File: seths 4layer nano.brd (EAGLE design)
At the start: 20.9 x 51.1 mm, 30 parts, among them IC1 FT232RL, J1 1981568-1, Q1 CSTCR6M00G53Z, X1 TSW-115-07-G-S, X2 TSW-115-07-G-S

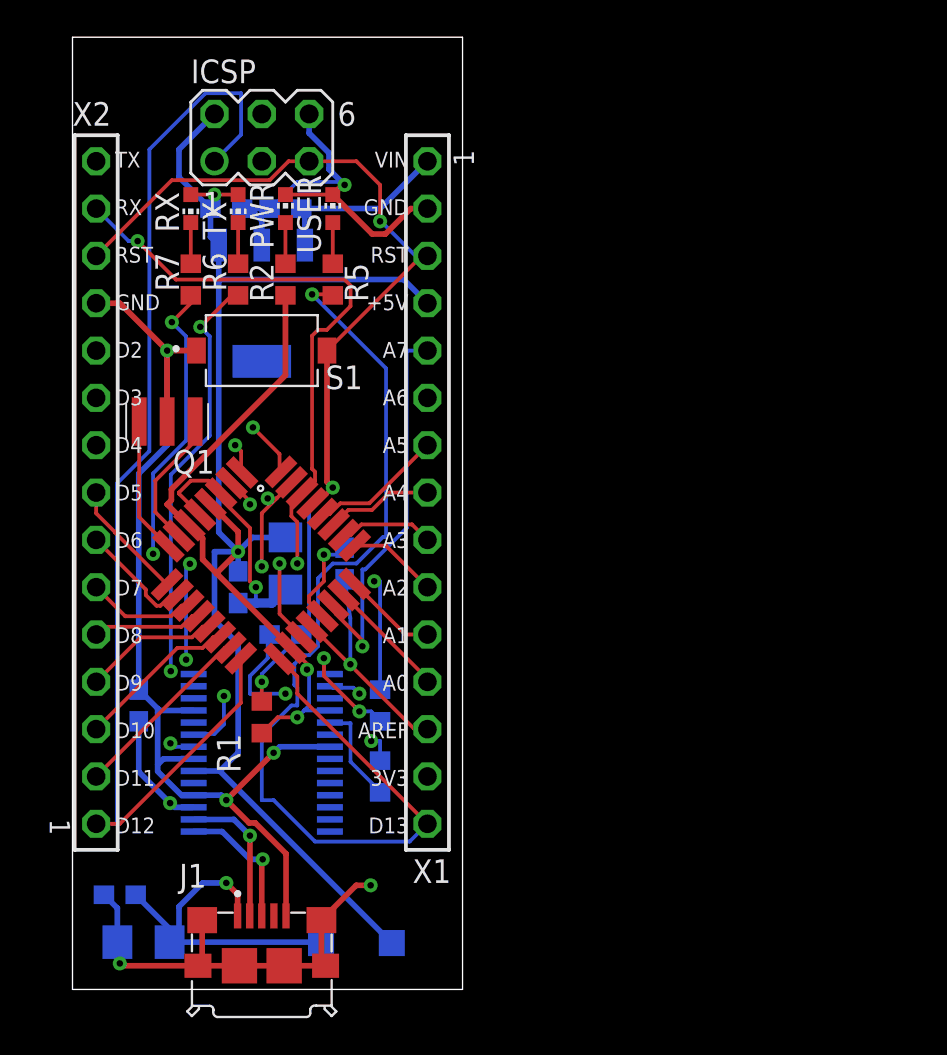
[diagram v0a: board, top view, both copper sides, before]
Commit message: Add files via upload
updating this since it hasn't been in a while.
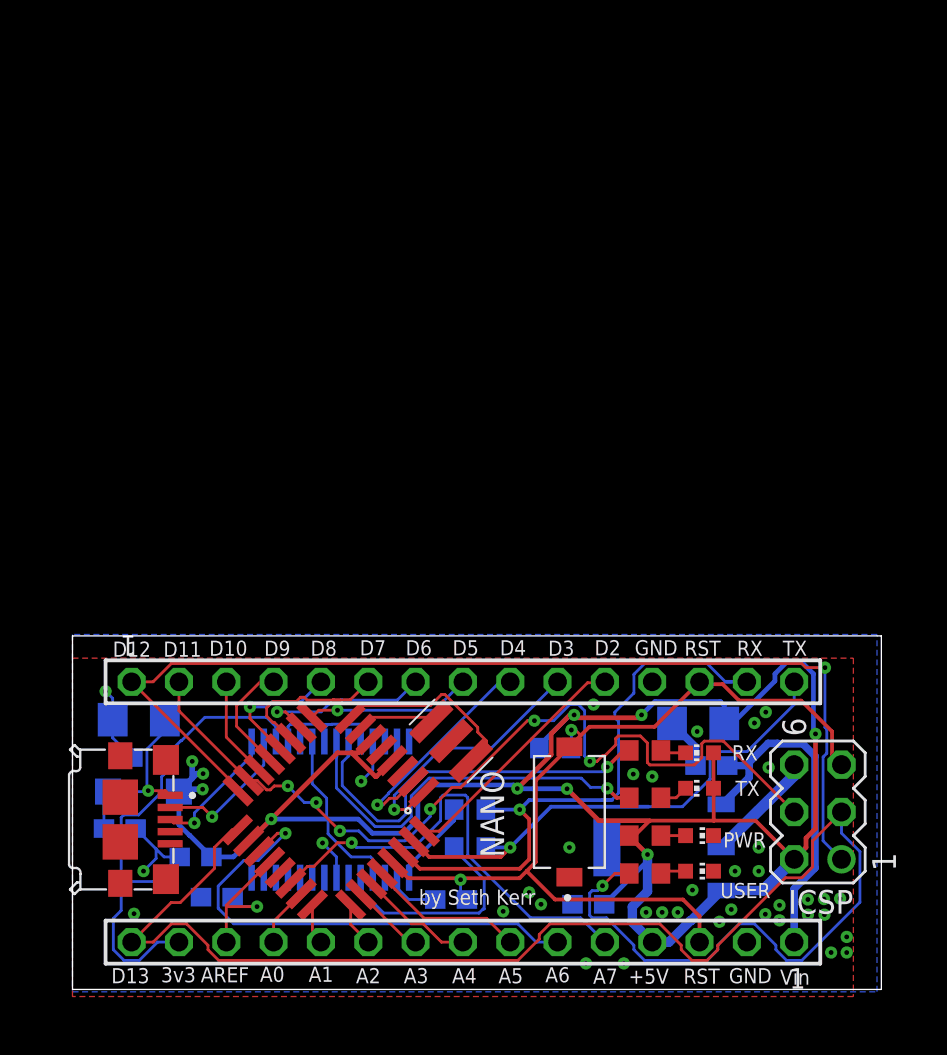
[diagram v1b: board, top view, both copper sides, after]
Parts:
- U1: device UA78M05CDCYR:DCY4 -> UA78M05CDCYR:DCY4-L
- moved ICSP 46.9 mm to (40.0, 9.53), turned to 90 degrees
- moved USER 40.6 mm to (33.7, 6.35), turned to 270 degrees
- moved PWR 40.3 mm to (33.7, 8.26), turned to 270 degrees
- moved RX 40.0 mm to (33.7, 12.7), turned to 90 degrees
- moved TX 39.8 mm to (33.7, 10.8), turned to 90 degrees
- moved C7 37.6 mm to (34.3, 12.0)
- moved U1 36.3 mm to (31.8, 7.62), turned to 270 degrees
- moved R5 36.0 mm to (30.7, 6.22), turned to 180 degrees
- moved R2 35.5 mm to (30.7, 8.26), turned to 180 degrees
- moved R6 35.4 mm to (30.7, 10.3), turned to 0 degrees
- moved R7 35.1 mm to (30.7, 12.8), turned to 0 degrees
- moved C8 34.8 mm to (6.60, 7.11), turned to 0 degrees
- moved S1 29.8 mm to (26.7, 9.53), turned to 90 degrees
- moved C3 25.4 mm to (27.7, 4.57), turned to 0 degrees
- moved X1 24.2 mm to (21.0, 2.54), turned to 0 degrees
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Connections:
- net +5V: now also U1.3; no longer U1.1
- net GND: now also IC1.26
- net VIN: now also U1.1; no longer U1.3
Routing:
- net GND: track 122.5 -> 28.1 mm, vias 8 -> 38
- net D13/SCK: track 64.7 -> 82.3 mm
- net +5V: track 110.3 -> 126.9 mm, vias 4 -> 10
- net TX/D1: track 40.9 -> 27.5 mm, vias 3 -> 1
- net RX/D0: track 42.8 -> 31.8 mm, vias 3 -> 1
- net A6: track 16.6 -> 26.8 mm
- net VIN: track 9.86 -> 18.8 mm
- net VUSB: track 18.5 -> 9.77 mm
- net N$16: track 11.3 -> 2.86 mm, vias 2 -> 0
- net TXLED: track 29.1 -> 20.9 mm, vias 5 -> 1
- net RXLED: track 27.9 -> 21.2 mm, vias 3 -> 1
- net TX: track 5.48 -> 12.0 mm
- net 3V3: track 20.8 -> 26.1 mm, vias 1 -> 0
- net AREF: track 13.1 -> 8.45 mm
- net D12/MISO: track 61.3 -> 56.8 mm, vias 0 -> 1
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- added copper zone on layer 1, net GND
- added copper zone on layer 16, net GND
- removed copper zone on layer 15, net GND
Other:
- board size 20.9 x 51.1 mm -> 43.4 x 19 mm
- board text added: "+5V"
- board text added: "3v3"
- board text added: "A0"
- board text added: "A1"
- board text added: "A2"
- board text added: "A3"
- board text added: "A4"
- board text added: "A5"
- board text added: "A6"
- board text added: "A7"
- board text added: "AREF"
- board text added: "D10"
- board text added: "D11"
- board text added: "D12"
- board text added: "D13"
- board text added: "D2"
- board text added: "D3"
- board text added: "D4"
- board text added: "D5"
- board text added: "D6"
- board text added: "D7"
- board text added: "D8"
- board text added: "D9"
- board text added: "GND"
- board text added: "ICSP"
- board text added: "NANO"
- board text added: "PWR"
- board text added: "RST"
- board text added: "RX"
- board text added: "TX"
- board text added: "USER"
- board text added: "Vin"
- board text added: "by Seth Kerr"
- board text removed: "Design By Seth Kerr"
- board text removed: "TX RX RST GND D2 D3 D4 D5 D6 D7 D8 D9 D10 D11 D12"
- board text removed: "VIN GND RST +5V A7 A6 A5 A4 A3 A2 A1 A0 AREF 3V3 D13"
- board text removed: "in 2020"
